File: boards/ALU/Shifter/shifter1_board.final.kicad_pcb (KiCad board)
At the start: 4 copper layers, 65 x 100 mm, 847 parts

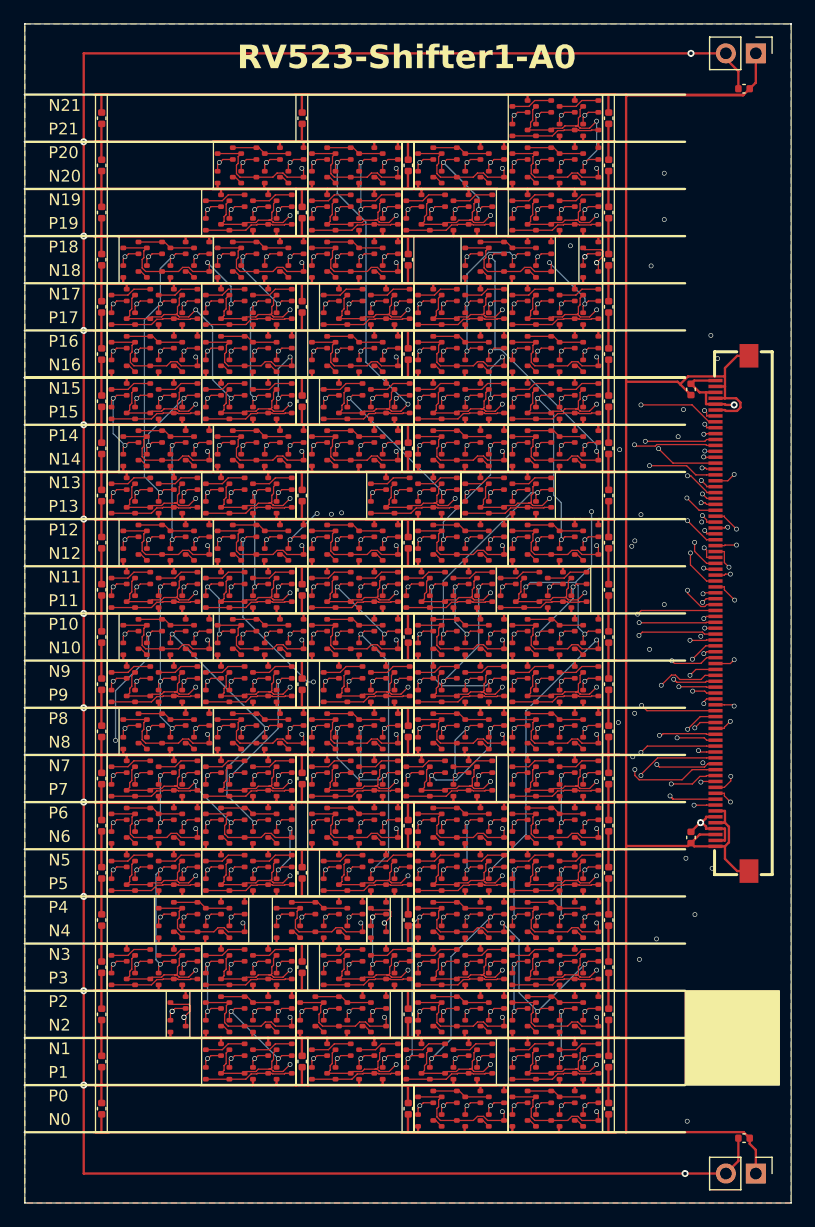
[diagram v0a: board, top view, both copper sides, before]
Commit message: Production files for shifter1
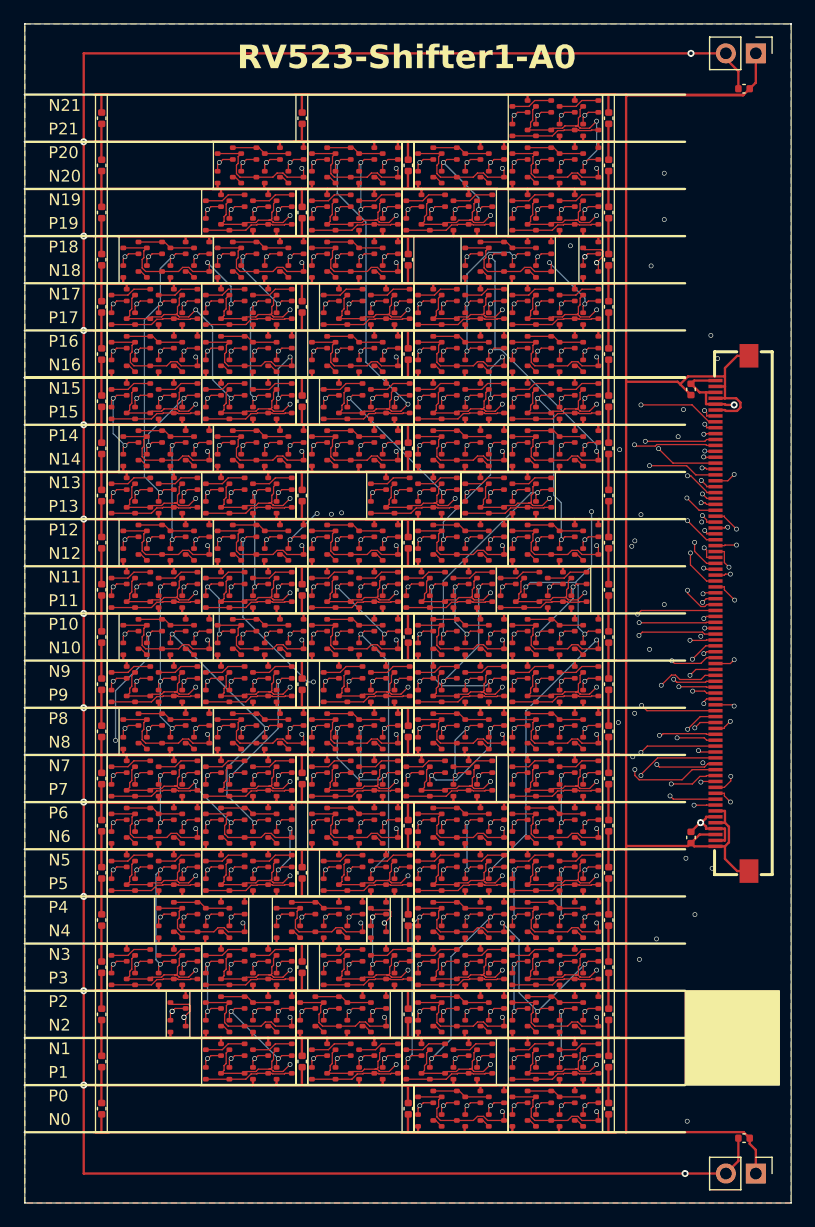
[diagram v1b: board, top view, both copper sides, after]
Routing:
- net GND: track 1780.0 -> 1743.8 mm
- net VDD: track 1855.3 -> 1820.5 mm
- net F.19: track 63.6 -> 62.0 mm
- net A.31: track 55.7 -> 54.5 mm
- net A.21: track 92.5 -> 91.6 mm
